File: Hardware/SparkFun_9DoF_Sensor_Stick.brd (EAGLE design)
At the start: 34.3 x 10.2 mm, 32 parts, among them U1 ITG-32001:1, U2 ADXL345", U3 3.3V/150mA, U4 HMC5883LSMD

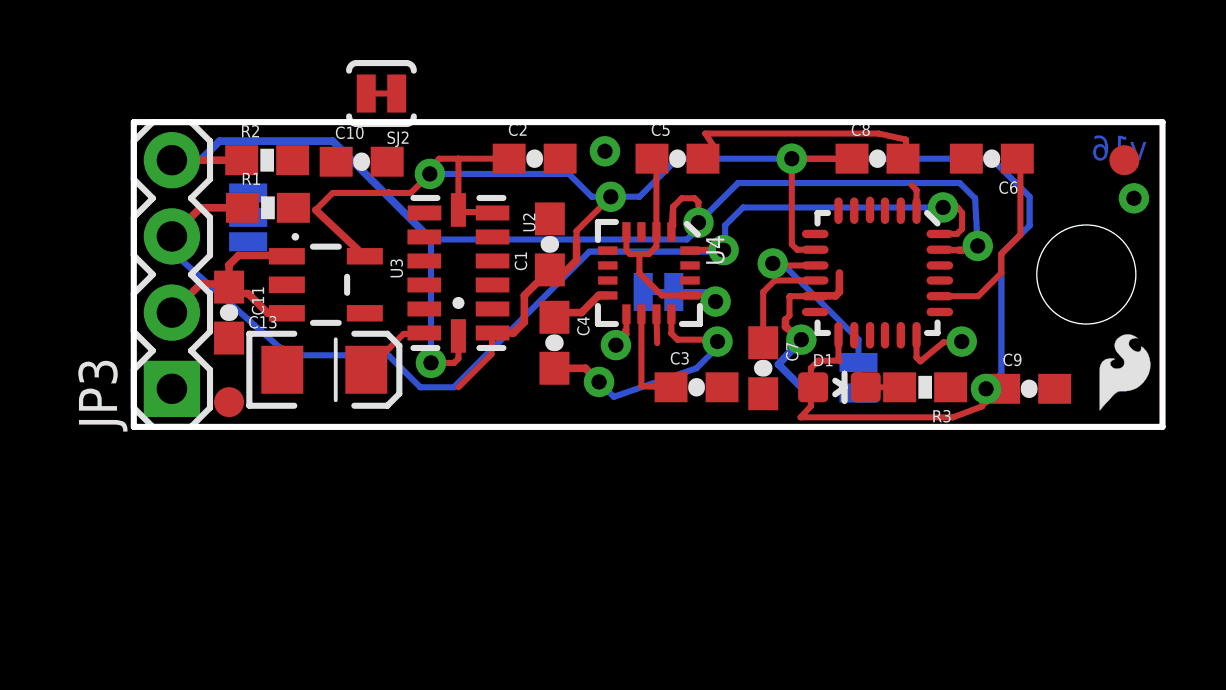
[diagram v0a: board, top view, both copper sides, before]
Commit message: Complete reroute-WIP
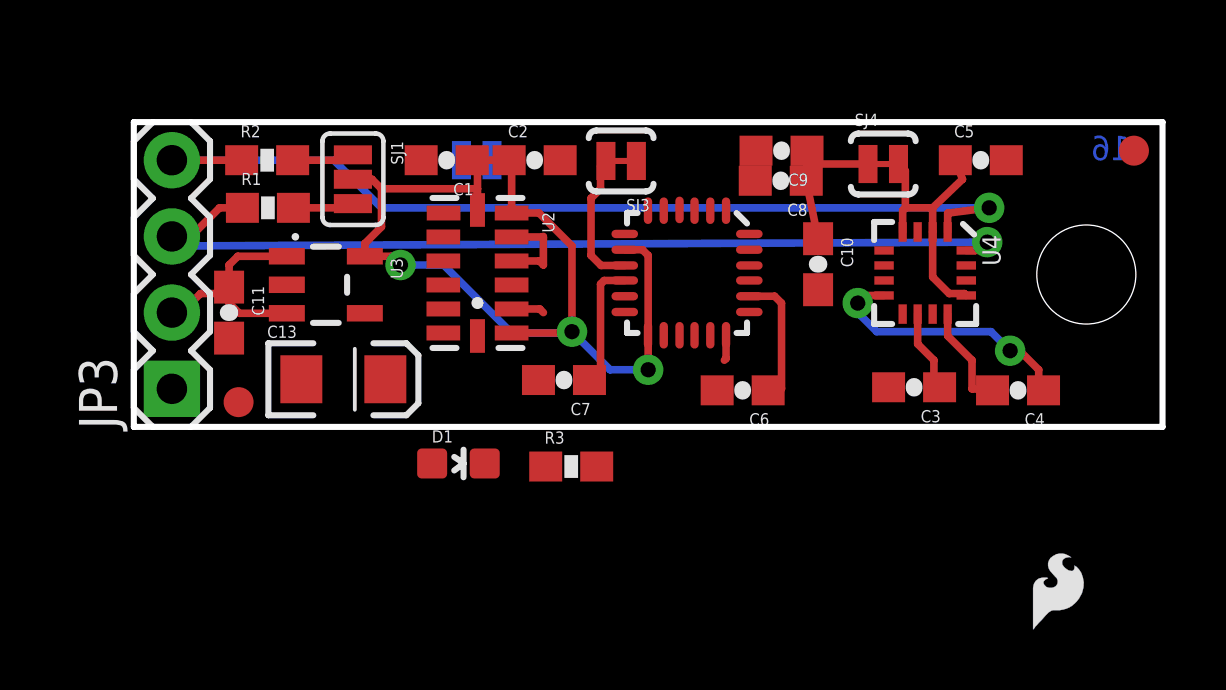
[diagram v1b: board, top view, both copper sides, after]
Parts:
- moved C10 15.6 mm to (22.8, 5.42), turned to 270 degrees
- moved C4 15.5 mm to (29.5, 1.22), turned to 180 degrees
- moved D1 13.0 mm to (10.8, -1.22)
- moved R3 12.1 mm to (14.6, -1.32), turned to 0 degrees
- moved C9 11.5 mm to (21.6, 9.21), turned to 180 degrees
- moved C6 11.3 mm to (20.3, 1.22)
- moved SJ3 10.7 mm to (16.2, 8.86), flipped to the top, turned to 180 degrees
- moved C5 10.1 mm to (28.2, 8.89)
- moved U4 9.21 mm to (26.4, 5.13)
- moved SJ4 8.62 mm to (25.0, 8.76), flipped to the top, turned to 0 degrees
- moved JP4 7.63 mm to (29.7, -7.11)
- moved C3 7.25 mm to (26.0, 1.32), turned to 180 degrees
- moved C7 6.65 mm to (14.3, 1.56), turned to 180 degrees
- moved U1 6.35 mm to (18.4, 5.13)
- moved C1 4.44 mm to (10.4, 8.89), turned to 180 degrees
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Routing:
- net 3.3V: track 67.5 -> 39.6 mm, vias 4 -> 3
- net GND: track 20.7 -> 5.19 mm, vias 5 -> 0
- net SCL: track 44.2 -> 32.2 mm, vias 3 -> 1
- net SDA: track 38.5 -> 31.0 mm, vias 2 -> 1
- net N$2: track 2.08 -> 8.87 mm, vias 0 -> 2
- net N$3: track 8.77 -> 3.51 mm, vias 2 -> 0
- net N$8: track 0.00 -> 2.08 mm
- net N$6: track 0.00 -> 2.04 mm
- net N$5: track 6.49 -> 4.47 mm
- net N$9: track 6.12 -> 4.62 mm, vias 1 -> 0
- net N$4: track 1.13 -> 0.00 mm
- net N$12: track 9.86 -> 9.04 mm, vias 1 -> 0
- net N$1: track 3.39 -> 2.77 mm
- net N$7: track 3.58 -> 4.20 mm
